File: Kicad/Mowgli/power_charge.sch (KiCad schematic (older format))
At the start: 28 parts, among them J2 Charge, J3 POWER, Q4 N06N-HIGH, Q4 N06N-LOW, SW1 Power Switch, U10 LM5109MA

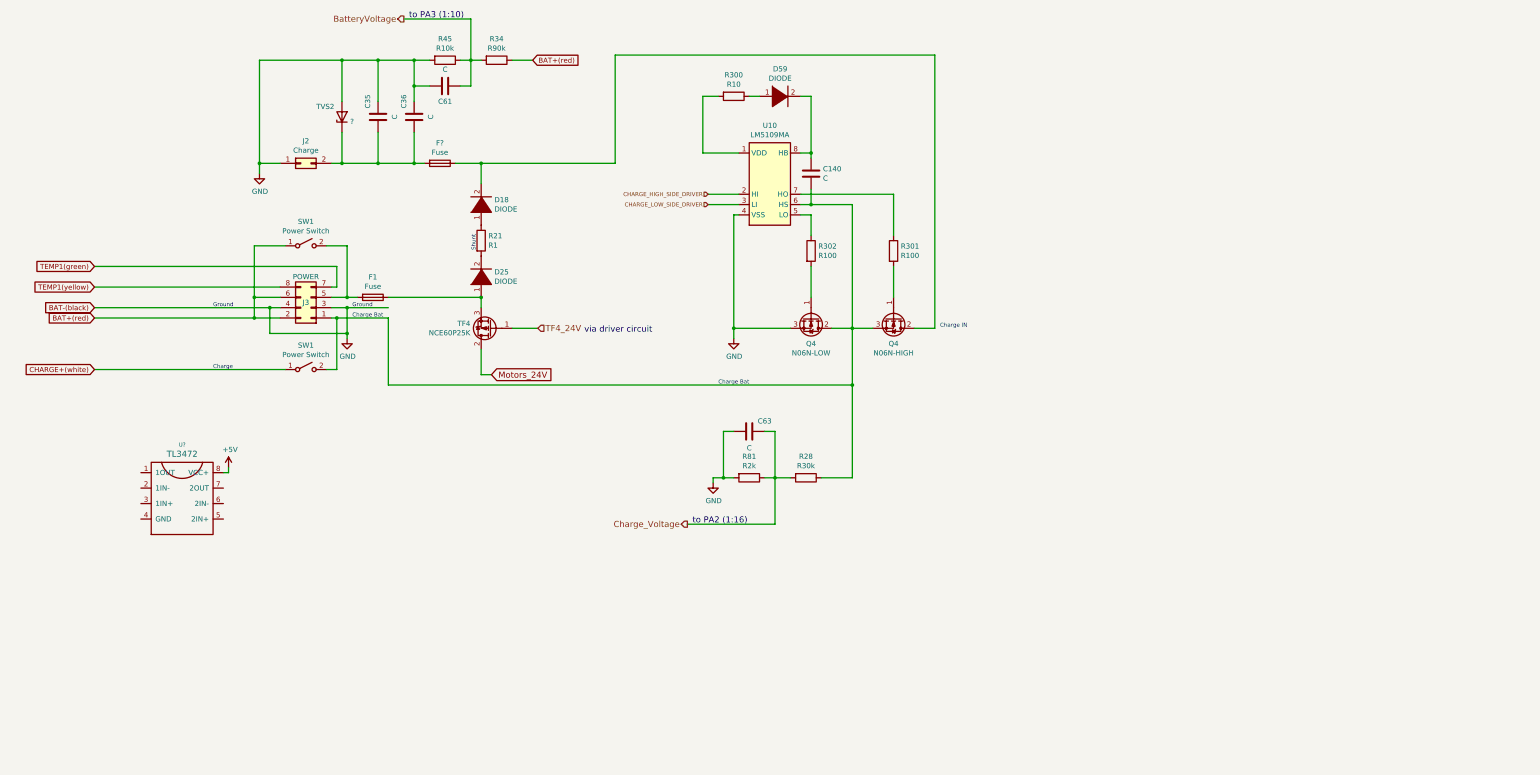
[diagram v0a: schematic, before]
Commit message: updated kicad
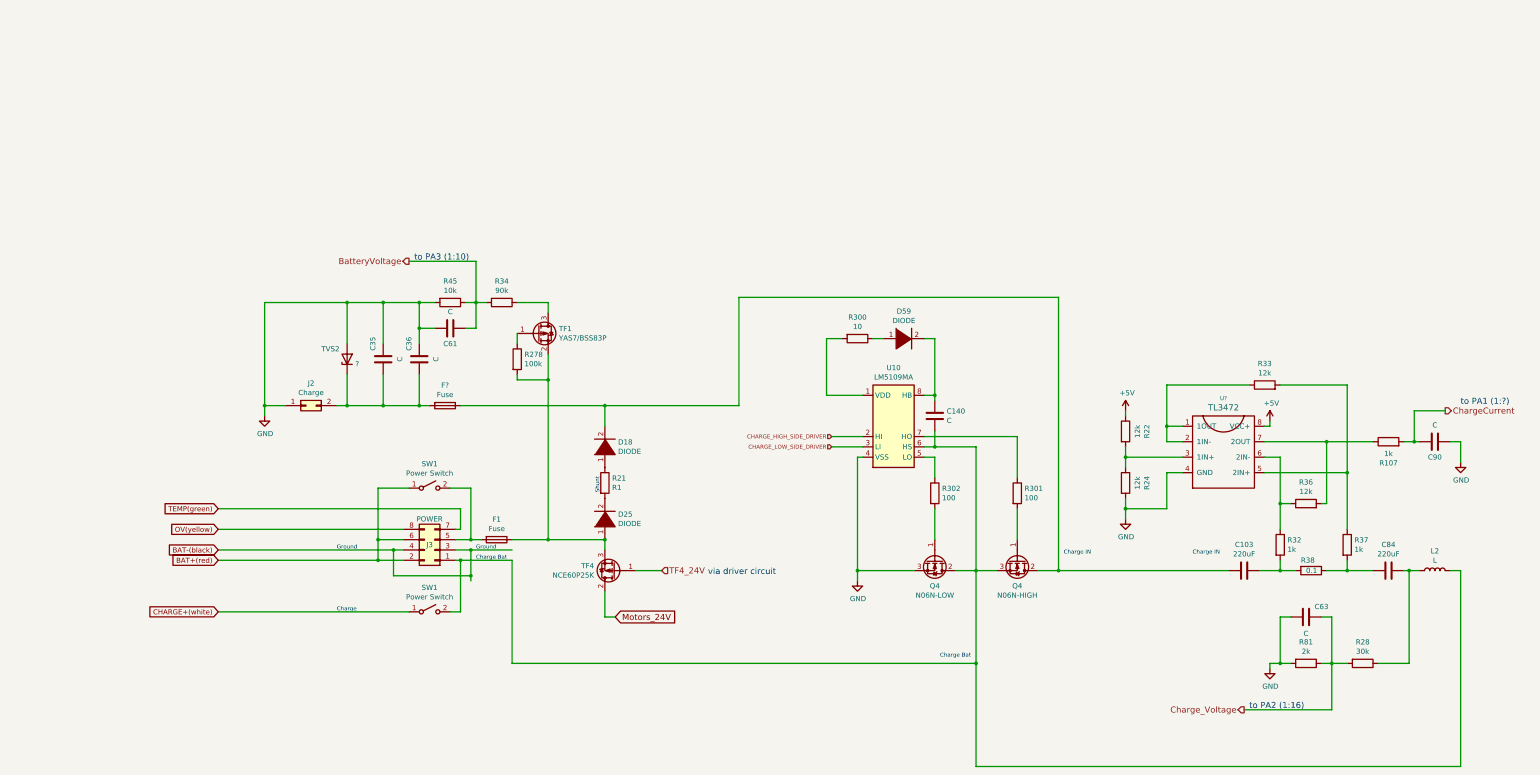
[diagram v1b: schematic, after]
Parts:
- added C103, C84: 220uF, symbol Device:C
- added C90: C, symbol Device:C
- added L2: L, symbol Device:L
- added R107, R32, R37: 1k, symbol Device:R
- added R22, R24, R33, R36: 12k, symbol Device:R
- added R278: 100k, symbol Device:R
- added R38: 0.1, symbol Device:R
- added TF1: YAS7/BSS83P, Package_TO_SOT_SMD:SOT-23, symbol Transistor_FET:AO3401A
- R28: value R30k -> 30k
- R300: value R10 -> 10
- R301, R302: value R100 -> 100
- R34: value R90k -> 90k
- R45: value R10k -> 10k
- R81: value R2k -> 2k
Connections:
- net +5V: now also R22.1
- net BAT+(red): no longer R34.1
- net GND: now also U?.4 (GND), C90.1, R24.2; no longer J3.3 (Pin_3), J3.4 (Pin_4)
- net at C140.2, J3.1 (Pin_1), Q4.2 (D)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: now also L2.2; no longer R28.1
- net at D18.2 (A), F?.1, Q4.2 (D): now also C103.2
- net at D25.1 (K), F1.1, TF4.3 (S): now also R278.2, TF1.2 (S)
- net at U?.1 (1OUT): now also U?.2 (1IN-), R33.1
- net at U?.3 (1IN+): now also R22.2, R24.1
- net at U?.5 (2IN+): now also R33.2, R37.1
- net at U?.6 (2IN-): now also R32.1, R36.1
- net at U?.7 (2OUT): now also R107.1, R36.2
- net TEMP1(green) renamed TEMP(green)
- net TEMP1(yellow) renamed OV(yellow)
- new net: R34.1, TF1.3 (D)
- new net: C84.1, L2.1, R28.1
- new net: C84.2, R37.2, R38.1
- new net: C103.1, R32.2, R38.2
- new net: R278.1, TF1.1 (G)
- new net BAT-(black): J3.3 (Pin_3), J3.4 (Pin_4)
- new net ChargeCurrent: C90.2, R107.2
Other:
- note added: "to PA1 (1:?)"
- moved on the sheet: C140, C35, C36, C61, C63, D18, D25, D59, F1, F?, J2, J3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
